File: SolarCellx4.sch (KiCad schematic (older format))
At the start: 0 parts

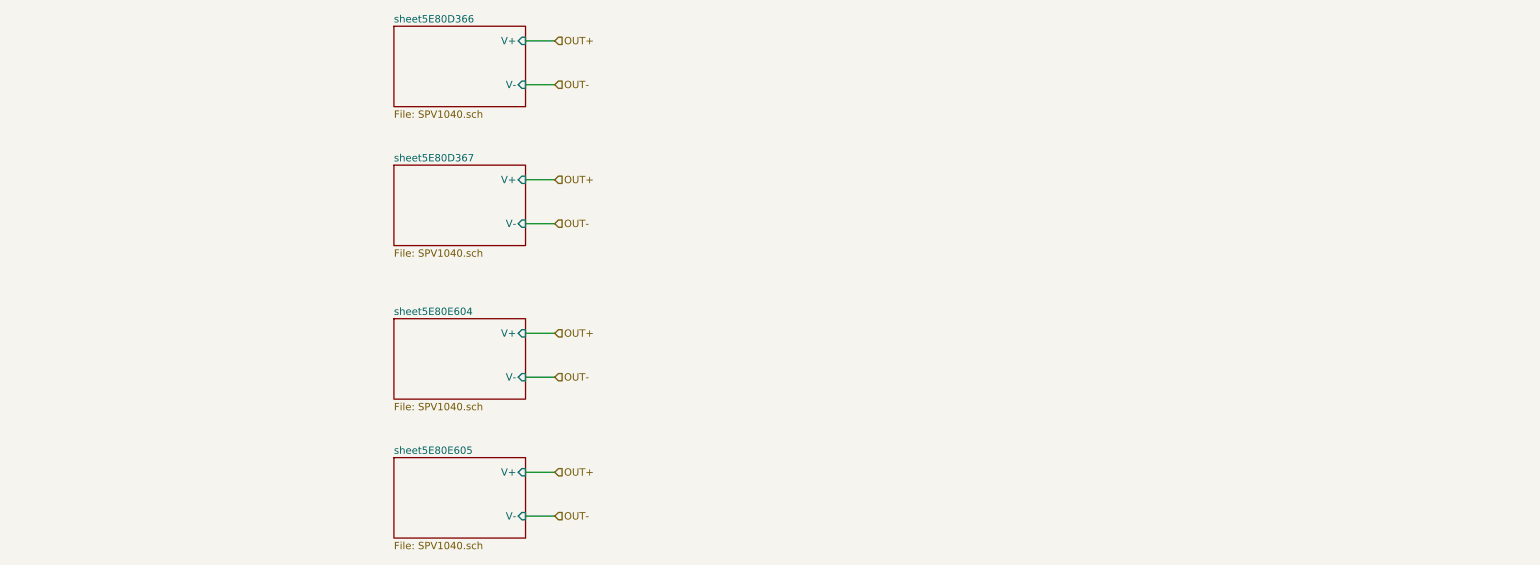
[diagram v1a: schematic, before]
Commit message: finish
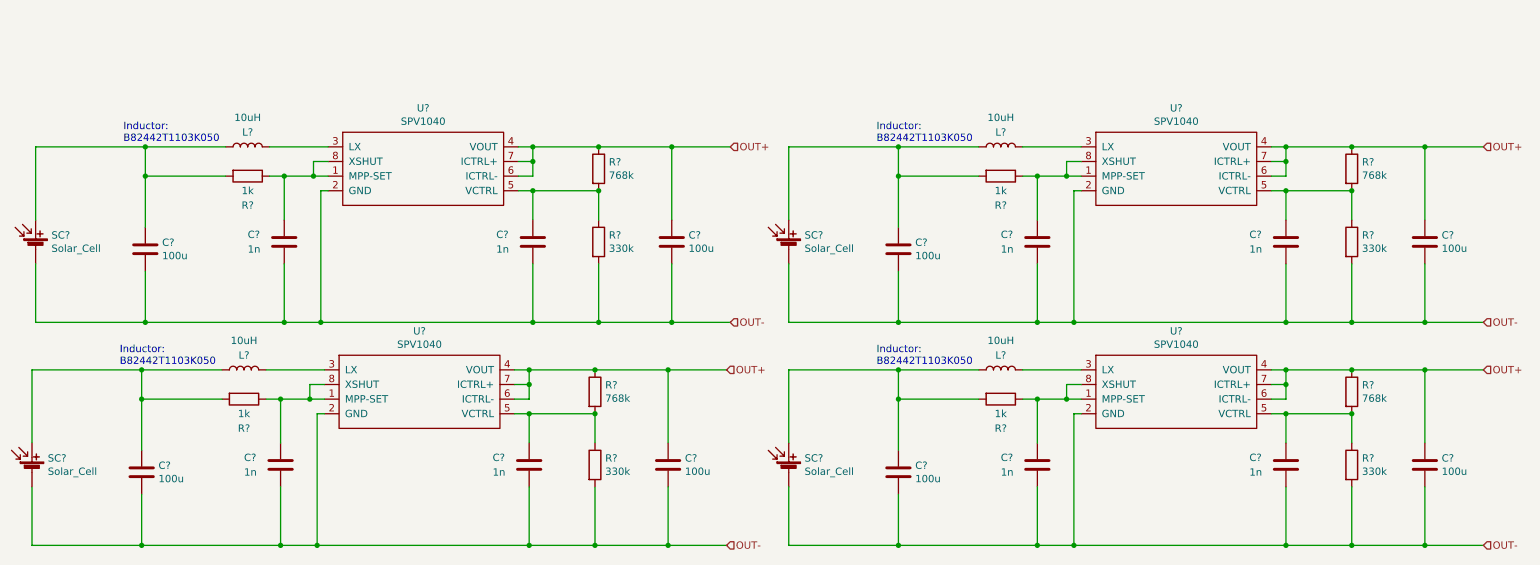
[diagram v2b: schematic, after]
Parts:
- added C? (x8): 1n, symbol Device:C
- added C? (x8): 100u, symbol Main-rescue:C-Device
- added L? (x4): 10uH, symbol Main-rescue:L-Device
- added R? (x4): 330k, symbol Device:R
- added R? (x4): 768k, symbol Device:R
- added R? (x4): 1k, symbol Main-rescue:R-Device
- added SC? (x4): Solar_Cell, symbol Device:Solar_Cell
- added U? (x4): SPV1040, symbol Main-rescue:SPV1040-CustomSymbols
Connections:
- net OUT+: now also C?.1, C?.1, C?.1, C?.1, R?.1, R?.1, R?.1, R?.1, U?.4 (VOUT), U?.4 (VOUT), U?.4 (VOUT), U?.4 (VOUT), U?.6 (ICTRL-), U?.6 (ICTRL-), U?.6 (ICTRL-), U?.6 (ICTRL-), U?.7 (ICTRL+), U?.7 (ICTRL+), U?.7 (ICTRL+), U?.7 (ICTRL+)
- net OUT-: now also C?.2, C?.2, C?.2, C?.2, C?.2, C?.2, C?.2, C?.2, C?.2, C?.2, C?.2, C?.2, C?.2, C?.2, C?.2, C?.2, R?.2, R?.2, R?.2, R?.2, SC?.2 (-), SC?.2 (-), SC?.2 (-), SC?.2 (-), U?.2 (GND), U?.2 (GND), U?.2 (GND), U?.2 (GND)
- new net: C?.1, L?.1, R?.2, SC?.1 (+) (x4)
- new net: C?.1, R?.1, R?.2, U?.5 (VCTRL) (x4)
- new net: C?.1, R?.1, U?.1 (MPP-SET), U?.8 (XSHUT) (x4)
- new net: L?.2, U?.3 (LX) (x4)
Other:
- note added: "Inductor:\nB82442T1103K050"
